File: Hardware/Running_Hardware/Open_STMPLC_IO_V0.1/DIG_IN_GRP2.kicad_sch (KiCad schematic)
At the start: 66 parts, among them J16 Screw_Terminal_01x02, J17 Screw_Terminal_01x02, J18 Screw_Terminal_01x02, J19 Screw_Terminal_01x02, J20 Screw_Terminal_01x02, J3 Screw_Terminal_01x02, U12 6N137, U20 6N137, U21 6N137, U22 6N137, U23 6N137, U24 6N137

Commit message: New DXF update
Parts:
- J16, J17, J18, J19, J20, J3: footprint TerminalBlock_Phoenix:TerminalBlock_Phoenix_MKDS-1,5-2_1x02_P5.00mm_Horizontal -> TerminalBlock_Phoenix:TerminalBlock_Phoenix_MKDS-1-2-3.81_1x02_P3.81mm_Horizontal
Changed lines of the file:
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@@
 			)
 		)
-		(property "Footprint" "TerminalBlock_Phoenix:TerminalBlock_Phoenix_MKDS-1,5-2_1x02_P5.00mm_Horizontal"
+		(property "Footprint" "TerminalBlock_Phoenix:TerminalBlock_Phoenix_MKDS-1-2-3.81_1x02_P3.81mm_Horizontal"
 			(at 203.2 128.27 0)
 			(effects
@@
 			)
 		)
-		(property "Footprint" "TerminalBlock_Phoenix:TerminalBlock_Phoenix_MKDS-1,5-2_1x02_P5.00mm_Horizontal"
+		(property "Footprint" "TerminalBlock_Phoenix:TerminalBlock_Phoenix_MKDS-1-2-3.81_1x02_P3.81mm_Horizontal"
 			(at 114.3 124.46 0)
 			(effects
@@
 			)
 		)
-		(property "Footprint" "TerminalBlock_Phoenix:TerminalBlock_Phoenix_MKDS-1,5-2_1x02_P5.00mm_Horizontal"
+		(property "Footprint" "TerminalBlock_Phoenix:TerminalBlock_Phoenix_MKDS-1-2-3.81_1x02_P3.81mm_Horizontal"
 			(at 22.86 50.8 0)
 			(effects
@@
 			)
 		)
-		(property "Footprint" "TerminalBlock_Phoenix:TerminalBlock_Phoenix_MKDS-1,5-2_1x02_P5.00mm_Horizontal"
+		(property "Footprint" "TerminalBlock_Phoenix:TerminalBlock_Phoenix_MKDS-1-2-3.81_1x02_P3.81mm_Horizontal"
 			(at 114.3 49.53 0)
 			(effects
@@
 			)
 		)
-		(property "Footprint" "TerminalBlock_Phoenix:TerminalBlock_Phoenix_MKDS-1,5-2_1x02_P5.00mm_Horizontal"
+		(property "Footprint" "TerminalBlock_Phoenix:TerminalBlock_Phoenix_MKDS-1-2-3.81_1x02_P3.81mm_Horizontal"
 			(at 203.2 49.53 0)
 			(effects
@@
 			)
 		)
-		(property "Footprint" "TerminalBlock_Phoenix:TerminalBlock_Phoenix_MKDS-1,5-2_1x02_P5.00mm_Horizontal"
+		(property "Footprint" "TerminalBlock_Phoenix:TerminalBlock_Phoenix_MKDS-1-2-3.81_1x02_P3.81mm_Horizontal"
 			(at 22.86 125.73 0)
 			(effects

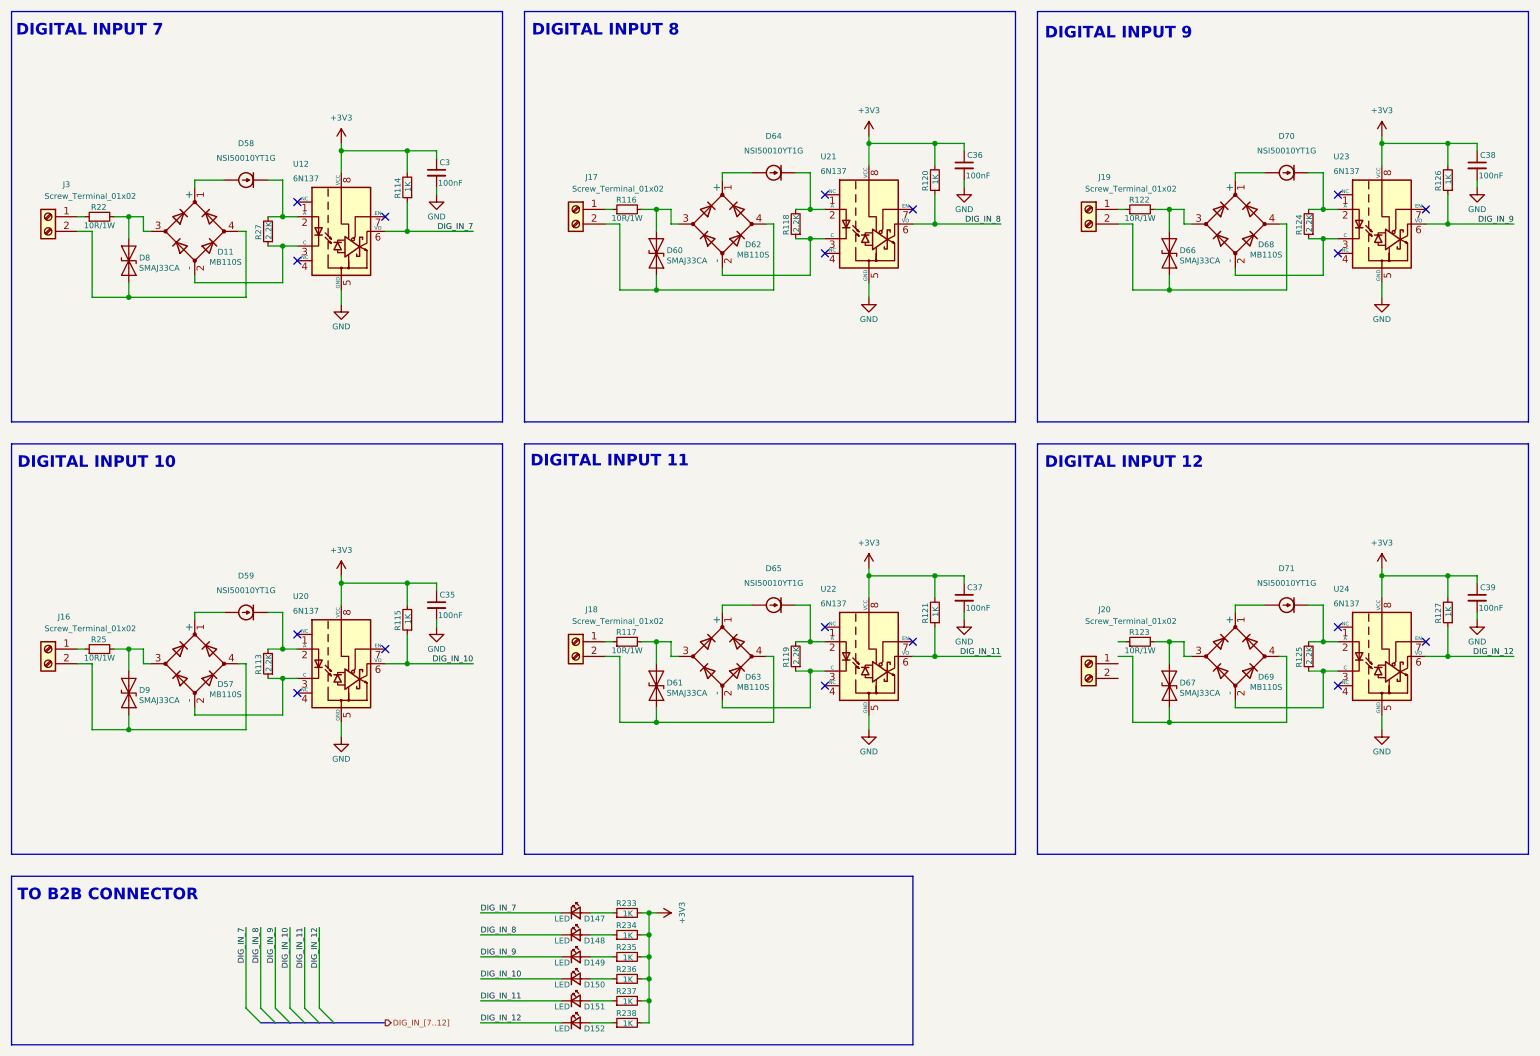
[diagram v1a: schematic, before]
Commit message: Rule areas creation
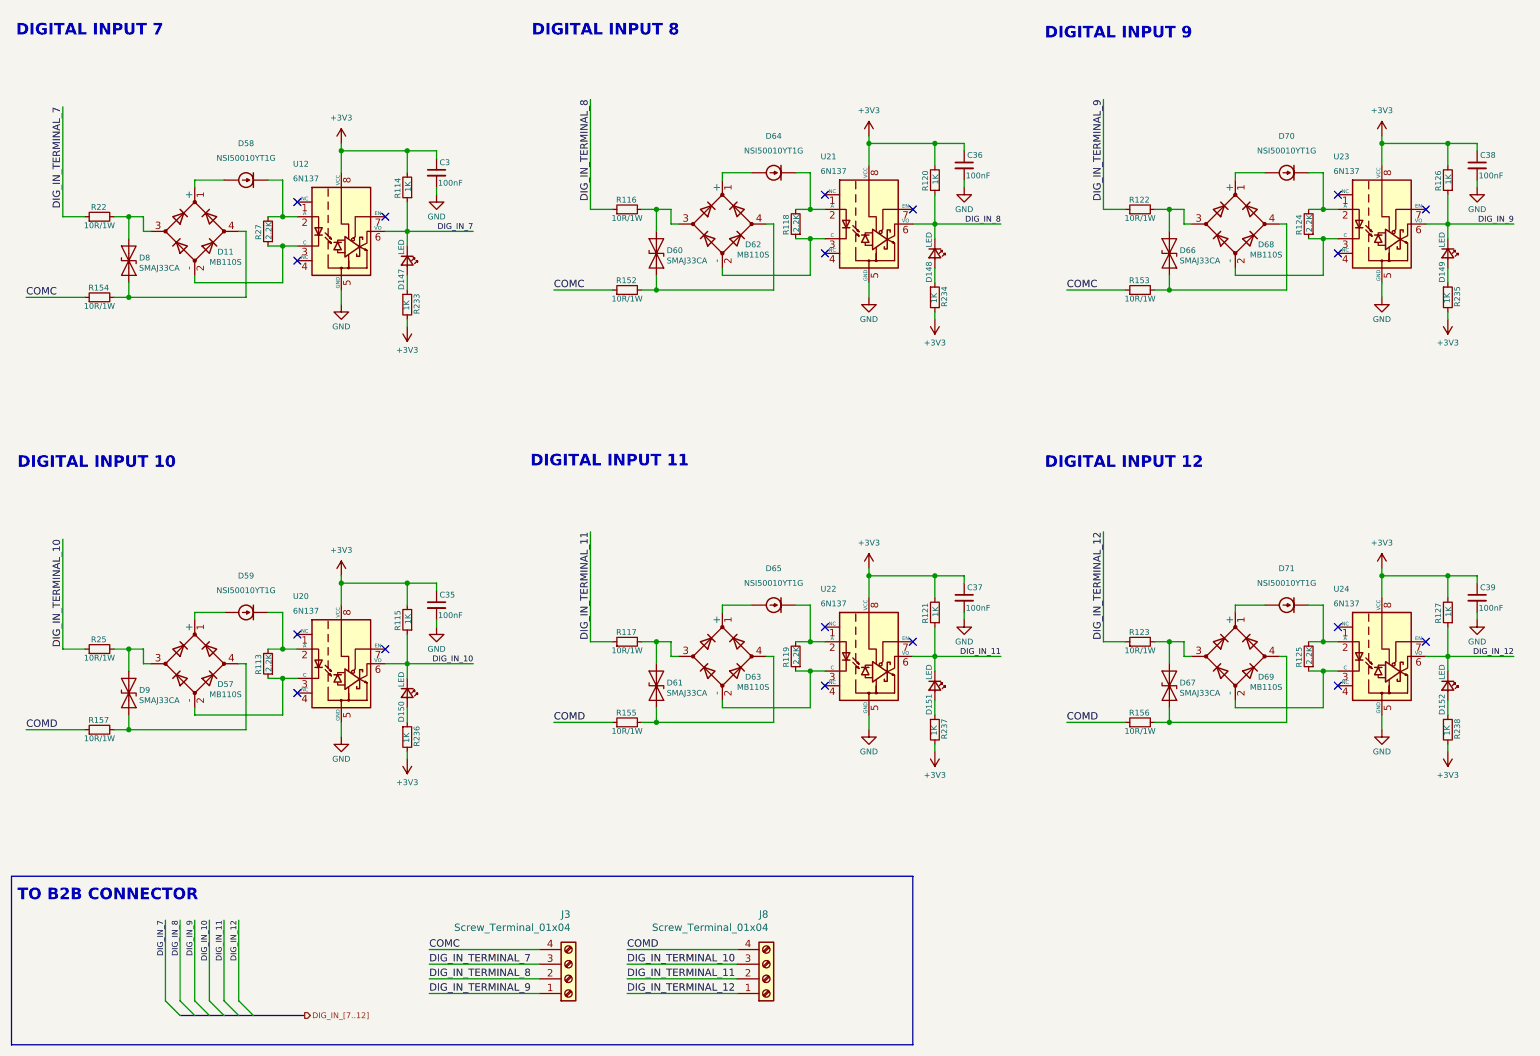
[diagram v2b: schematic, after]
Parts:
- removed J16, J17, J18, J19, J20, J3: Screw_Terminal_01x02, TerminalBlock_Phoenix:TerminalBlock_Phoenix_MKDS-1-2-3.81_1x02_P3.81mm_Horizontal, symbol Connector:Screw_Terminal_01x02
- added J3, J8: Screw_Terminal_01x04, TerminalBlock_Phoenix:TerminalBlock_Phoenix_MKDS-1-4-3.81_1x04_P3.81mm_Horizontal, symbol Connector:Screw_Terminal_01x04
- added R152, R153, R154, R155, R156, R157: 10R/1W, Resistor_SMD:R_0603_1608Metric_Pad0.98x0.95mm_HandSolder, symbol Device:R_Small
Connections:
- net at D57.4, D9.2 (A2): now also R157.2
- net at D67.2 (A2), D69.4: now also R156.2
- net at D60.2 (A2), D62.4: now also R152.2
- net at D61.2 (A2), D63.4: now also R155.2
- net at D66.2 (A2), D68.4: now also R153.2
- net DIG_IN_TERMINAL_8: now reaches R116.1
- net DIG_IN_TERMINAL_8: now also J3.2 (Pin_2)
- net DIG_IN_TERMINAL_12: now reaches R123.1
- net DIG_IN_TERMINAL_12: now also J8.1 (Pin_1)
- net DIG_IN_TERMINAL_11: now reaches R117.1
- net DIG_IN_TERMINAL_11: now also J8.2 (Pin_2)
- net DIG_IN_TERMINAL_7: now reaches R22.1
- net DIG_IN_TERMINAL_7: now also J3.3 (Pin_3)
- net at D11.4, D8.2 (A2): now also R154.2
- net DIG_IN_TERMINAL_9: now reaches R122.1
- net DIG_IN_TERMINAL_9: now also J3.1 (Pin_1)
- net DIG_IN_TERMINAL_10: now reaches R25.1
- net DIG_IN_TERMINAL_10: now also J8.3 (Pin_3)
- new net COMC: J3.4 (Pin_4), R152.1, R153.1, R154.1
- new net COMD: J8.4 (Pin_4), R155.1, R156.1, R157.1
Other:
- moved on the sheet: D147, D148, D149, D150, D151, D152, R233, R234, R235, R236, R237, R238
